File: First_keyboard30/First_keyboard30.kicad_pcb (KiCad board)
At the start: 2 copper layers, 238.1 x 57.2 mm, 75 parts, among them SW1 RESET_SW, SW10 KEY_SW, SW11 KEY_SW, SW12 KEY_SW, SW13 KEY_SW, SW14 KEY_SW, SW15 KEY_SW, SW16 KEY_SW, SW17 KEY_SW, SW18 KEY_SW, SW19 KEY_SW, SW2 KEY_SW, SW20 KEY_SW, SW21 KEY_SW, SW22 KEY_SW, SW23 KEY_SW, SW24 KEY_SW, SW25 KEY_SW, SW26 KEY_SW, SW27 KEY_SW, SW28 KEY_SW, SW29 KEY_SW, SW3 KEY_SW, SW30 KEY_SW, SW31 KEY_SW, SW32 KEY_SW, SW33 KEY_SW, SW34 KEY_SW, SW35 KEY_SW, SW4 KEY_SW, SW5 KEY_SW, SW6 KEY_SW, SW7 KEY_SW, SW8 KEY_SW, SW9 KEY_SW, U1 ProMicro

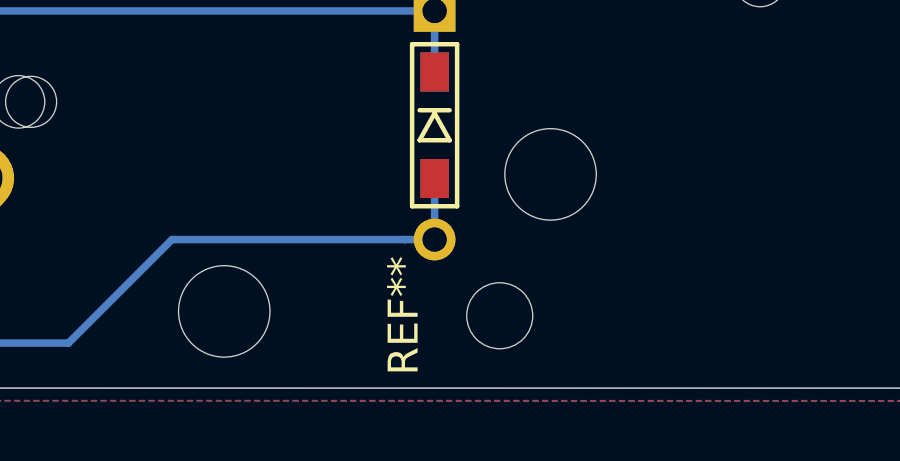
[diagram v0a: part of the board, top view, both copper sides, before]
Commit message: draw dxf
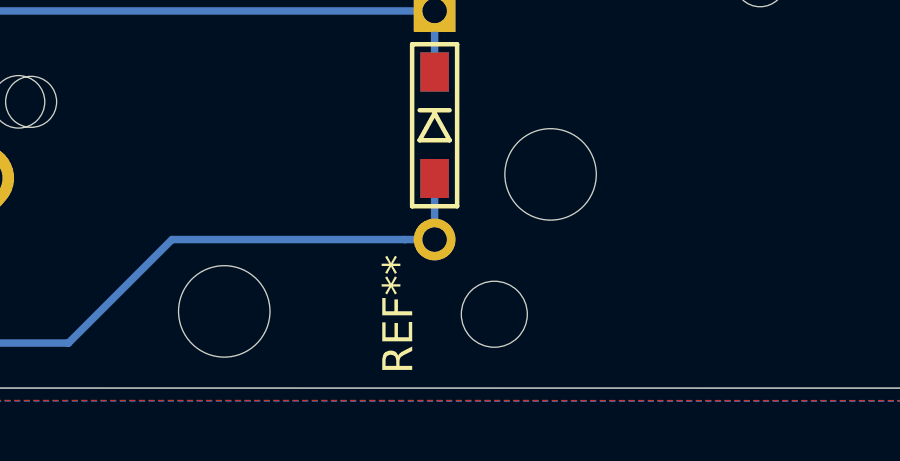
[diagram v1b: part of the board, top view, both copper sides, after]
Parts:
- moved REF** 0.19 mm to (245.4, 137.7)
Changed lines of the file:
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@@
       (padsonsilk false)
       (subtractmaskfromsilk false)
-      (outputformat 1)
+      (outputformat 3)
       (mirror false)
-      (drillshape 1)
+      (drillshape 0)
       (scaleselection 1)
-      (outputdirectory ""))
+      (outputdirectory "layout idea/"))
   )
   (net 0 "")
@@
   )
   (module MountingHole:MountingHole_2.2mm_M2 (layer F.Cu)
-    (at 245.56 137.76 90)
+    (at 245.38 137.71 90)
     (descr "Mounting Hole 2.2mm, no annular, M2")
     (tags "mounting hole 2.2mm no annular m2")
